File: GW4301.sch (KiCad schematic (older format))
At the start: 25 parts, among them J1 C64, U13 74LVC32, U19 XC6206P332MR

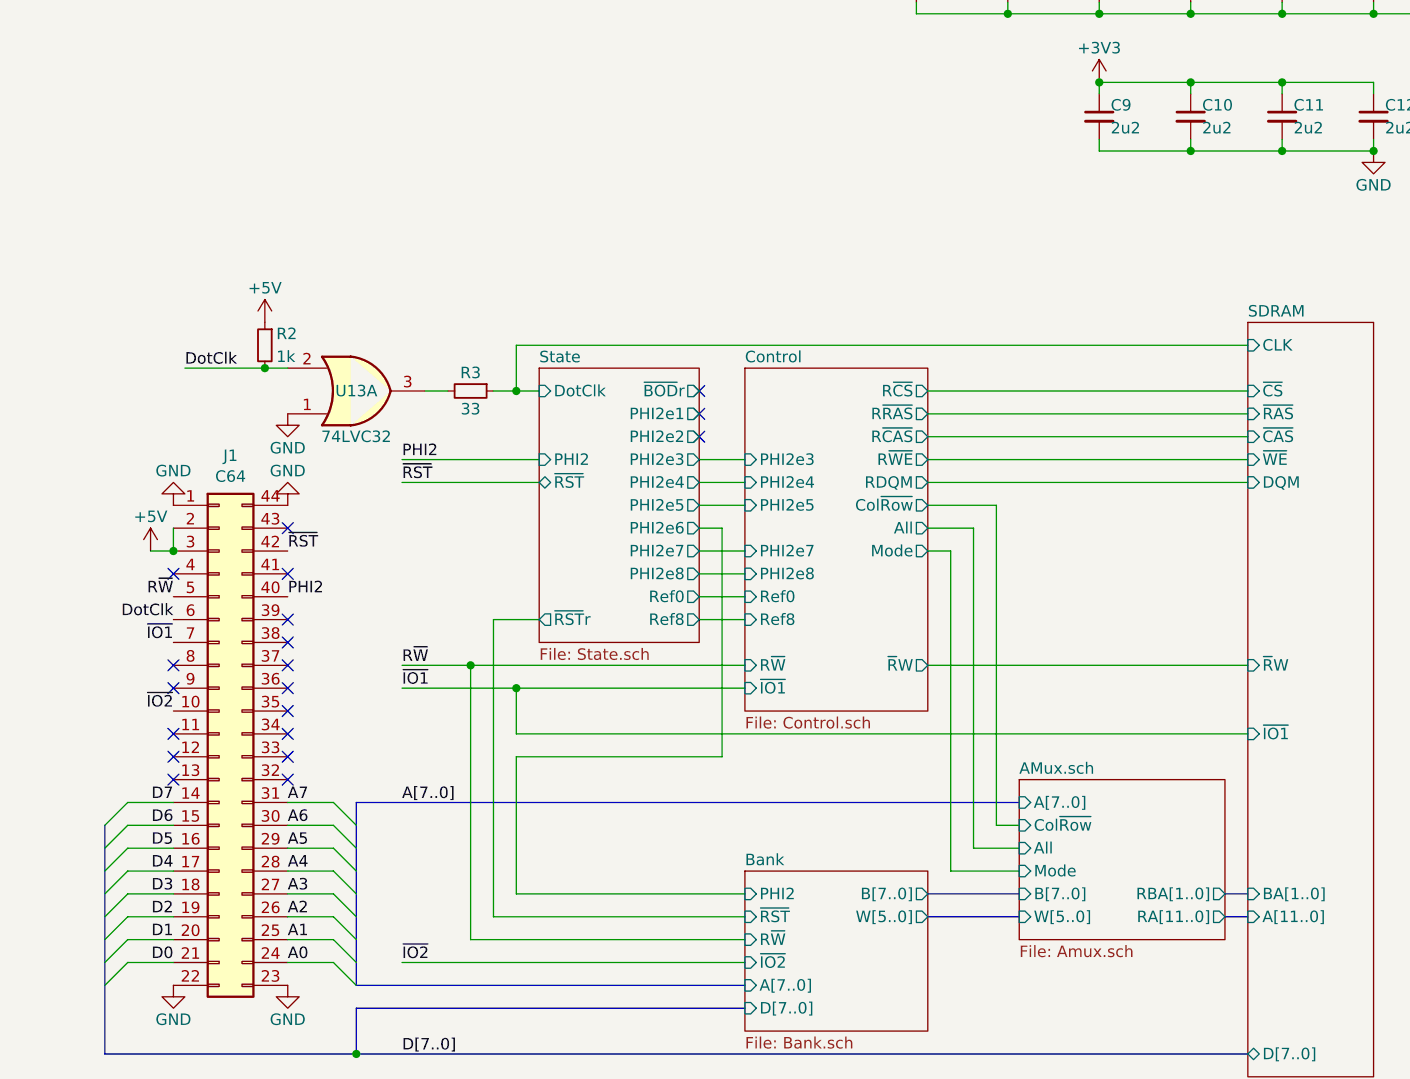
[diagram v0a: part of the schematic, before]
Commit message: PAL
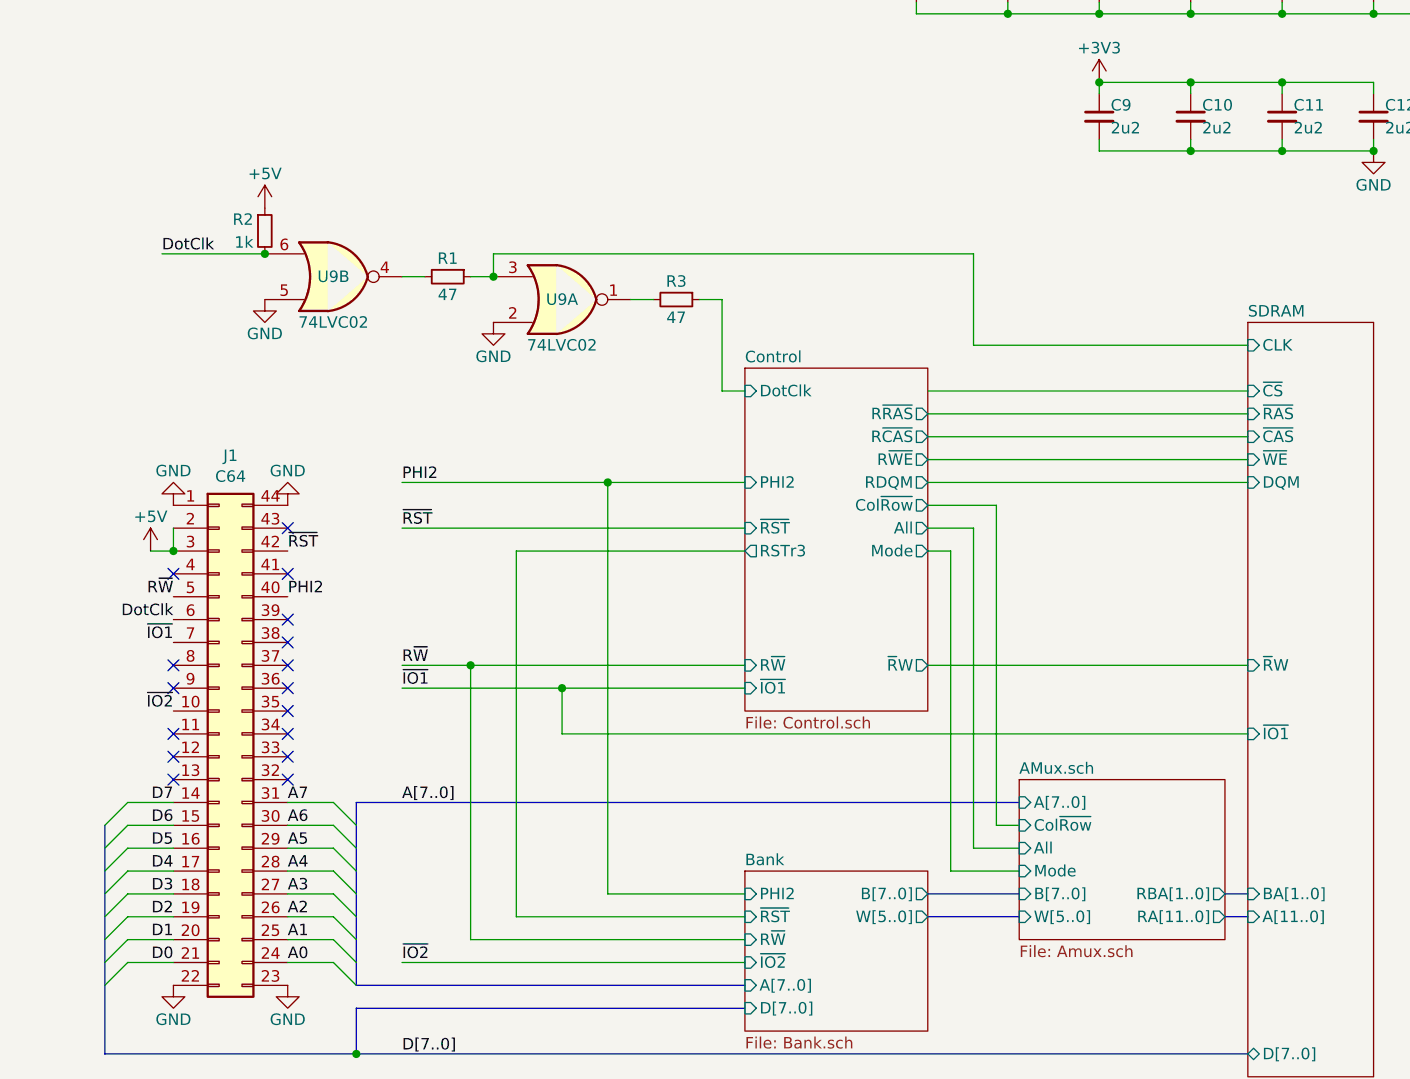
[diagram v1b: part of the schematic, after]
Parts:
- removed U13: 74LVC32, stdpads:TSSOP-14_4.4x5mm_P0.65mm, symbol 74xx:74LS32
- added R1: 47, stdpads:R_0603, symbol Device:R_Small
- added U9: 74LVC02, stdpads:TSSOP-14_4.4x5mm_P0.65mm, symbol 74xx:74LS02
- R3: value 33 -> 47
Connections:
- net DotClk: now also U9.6
- net GND: now also U9.2, U9.5
- net SDRAM/CLK: now also R1.1, U9.3; no longer R3.1
- net at R3.2: now also U9.1
- new net: R1.2, U9.4
- new net Control/DotClk: R3.1
- no-connect marks 19 -> 16
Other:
- moved on the sheet: R2
